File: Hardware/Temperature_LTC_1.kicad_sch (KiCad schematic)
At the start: 36 parts, among them J16 Conn_01x10

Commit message: New connectors jst_xh for low voltage side of bms
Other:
- title: (none) -> Battery Management System for a high power gokart battery
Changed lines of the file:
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@@
 	(generator_version "10.0")
 	(paper "A4")
+	(title_block
+		(title "Battery Management System for a high power gokart battery")
+	)
 	(junction
 		(at 129.54 100.33)

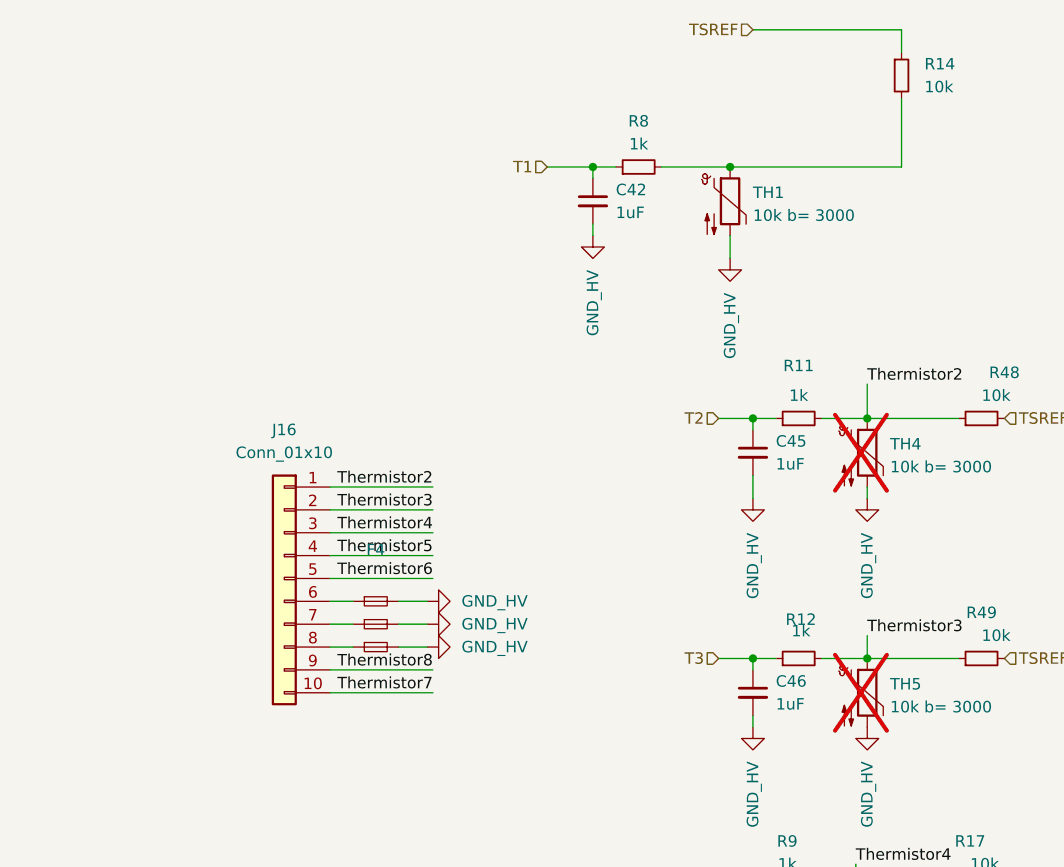
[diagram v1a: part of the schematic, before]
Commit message: No drc errors
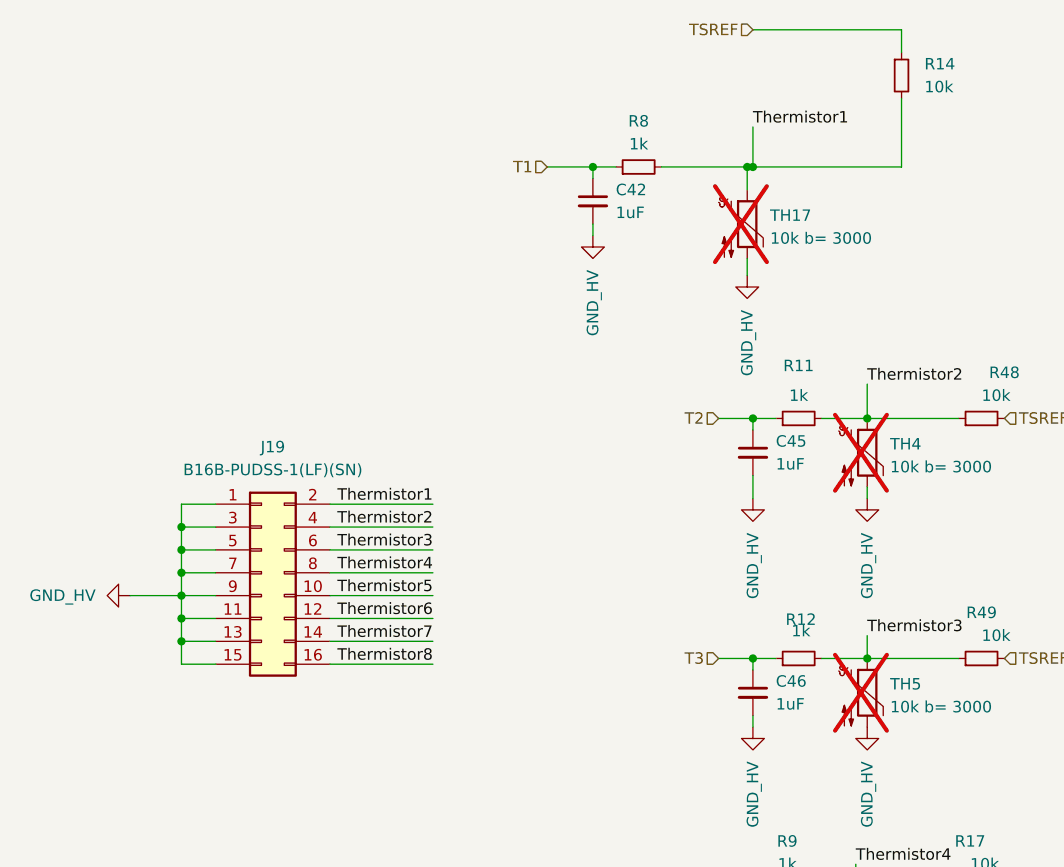
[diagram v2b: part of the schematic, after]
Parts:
- removed F4, F40, F41: 400mA, Fuse:Fuse_0805_2012Metric, symbol Device:Fuse_Small
- removed J16: Conn_01x10, footrpint:HARWIN_G125-MV11005L1P, symbol Connector_Generic:Conn_01x10
- removed TH1: 10k b= 3000, Resistor_SMD:R_0603_1608Metric_Pad0.98x0.95mm_HandSolder, symbol Device:Thermistor_NTC
- added J19: B16B-PUDSS-1(LF)(SN), Connector_JST:JST_PUD_B16B-PUDSS_2x08_P2.00mm_Vertical, symbol Connector_Generic:Conn_02x08_Odd_Even
- added TH17: 10k b= 3000, symbol Device:Thermistor_NTC
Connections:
- net GND_HV: now also J19.1 (Pin_1), J19.11 (Pin_11), J19.13 (Pin_13), J19.15 (Pin_15), J19.3 (Pin_3), J19.5 (Pin_5), J19.7 (Pin_7), J19.9 (Pin_9), TH17.2
- net Thermistor2: now also J19.4 (Pin_4)
- net Thermistor3: now also J19.6 (Pin_6)
- net Thermistor4: now also J19.8 (Pin_8)
- net Thermistor5: now also J19.10 (Pin_10)
- net Thermistor6: now also J19.12 (Pin_12)
- net Thermistor7: now also J19.14 (Pin_14)
- net Thermistor8: now also J19.16 (Pin_16)
- net Thermistor1: now reaches R14.2, R8.2
- net Thermistor1: now also J19.2 (Pin_2), TH17.1
